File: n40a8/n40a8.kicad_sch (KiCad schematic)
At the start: 92 parts, among them SW1 CPG151101S11-16, SW10 CPG151101S11-16, SW11 CPG151101S11-16, SW12 CPG151101S11-16, SW13 CPG151101S11-16, SW14 CPG151101S11-16, SW15 CPG151101S11-16, SW16 CPG151101S11-16, SW17 CPG151101S11-16, SW18 CPG151101S11-16, SW19 CPG151101S11-16, SW2 CPG151101S11-16, SW20 CPG151101S11-16, SW21 CPG151101S11-16, SW22 CPG151101S11-16, SW23 CPG151101S11-16, SW24 CPG151101S11-16, SW25 CPG151101S11-16, SW26 CPG151101S11-16, SW27 CPG151101S11-16, SW28 CPG151101S11-16, SW29 CPG151101S11-16, SW3 CPG151101S11-16, SW30 CPG151101S11-16, SW31 CPG151101S11-16, SW32 CPG151101S11-16, SW33 CPG151101S11-16, SW34 CPG151101S11-16, SW35 CPG151101S11-16, SW36 CPG151101S11-16, SW37 CPG151101S11-16, SW38 CPG151101S11-16, SW39 CPG151101S11-16, SW4 CPG151101S11-16, SW40 CPG151101S11-16, SW41 CPG151101S11-16, SW42 CPG151101S11-16, SW43 SW_RST, SW44 SW_PWR, SW5 CPG151101S11-16, SW6 CPG151101S11-16, SW7 CPG151101S11-16, SW8 CPG151101S11-16, SW9 CPG151101S11-16, U1 BLE-Micro-Pro-2, U2 TPS61221

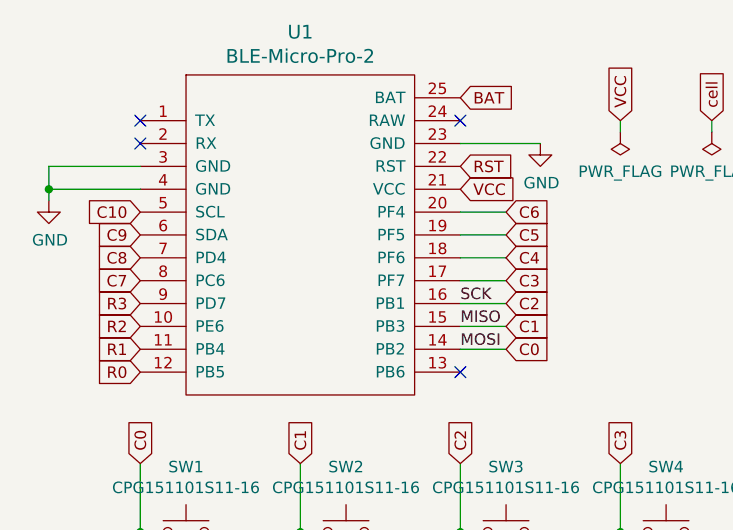
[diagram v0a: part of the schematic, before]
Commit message: revice for PCBA
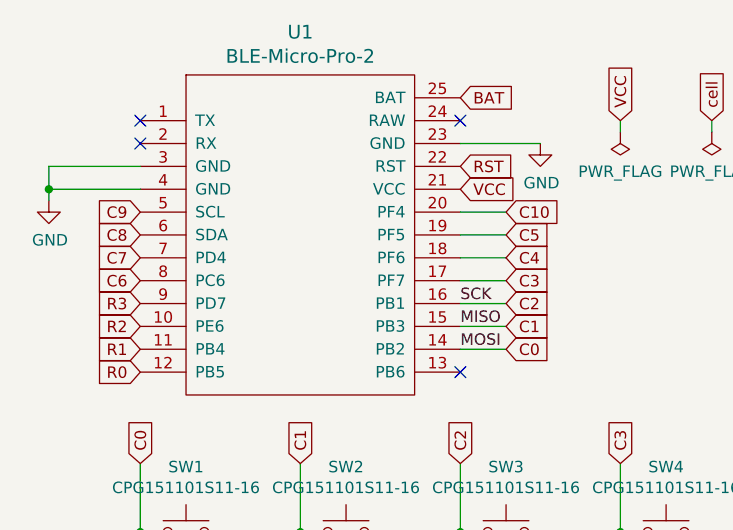
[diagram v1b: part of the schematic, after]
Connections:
- net C10: now also U1.20 (PF4); no longer U1.5 (SCL)
- net C6: now also U1.8 (PC6); no longer U1.20 (PF4)
- net C7: now also U1.7 (PD4); no longer U1.8 (PC6)
- net C8: now also U1.6 (SDA); no longer U1.7 (PD4)
- net C9: now also U1.5 (SCL); no longer U1.6 (SDA)
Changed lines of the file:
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@@
 	(global_label "C9"
 		(shape input)
-		(at 25.4 38.1 180)
-		(effects
-			(font
-				(size 1.27 1.27)
-			)
-			(justify right)
-		)
-		(property "Intersheetrefs" "${INTERSHEET_REFS}"
-			(at 25.4 38.1 0)
+		(at 25.4 35.56 180)
+		(effects
+			(font
+				(size 1.27 1.27)
+			)
+			(justify right)
+		)
+		(property "Intersheetrefs" "${INTERSHEET_REFS}"
+			(at 25.4 35.56 0)
 			(effects
 				(font
@@
 	(global_label "C7"
 		(shape input)
+		(at 25.4 40.64 180)
+		(effects
+			(font
+				(size 1.27 1.27)
+			)
+			(justify right)
+		)
+		(property "Intersheetrefs" "${INTERSHEET_REFS}"
+			(at 25.4 40.64 0)
+			(effects
+				(font
+					(size 1.27 1.27)
+				)
+				(hide yes)
+			)
+		)
+	)
+	(global_label "BAT"
+		(shape input)
+		(at 60.96 22.86 0)
+		(effects
+			(font
+				(size 1.27 1.27)
+			)
+			(justify left)
+		)
+		(property "Intersheetrefs" "${INTERSHEET_REFS}"
+			(at 60.96 22.86 0)
+			(effects
+				(font
+					(size 1.27 1.27)
+				)
+				(hide yes)
+			)
+		)
+	)
+	(global_label "VCC"
+		(shape input)
+		(at 78.74 25.4 90)
+		(effects
+			(font
+				(size 1.27 1.27)
+			)
+			(justify left)
+		)
+		(property "Intersheetrefs" "${INTERSHEET_REFS}"
+			(at 78.74 25.4 0)
+			(effects
+				(font
+					(size 1.27 1.27)
+				)
+				(hide yes)
+			)
+		)
+	)
+	(global_label "C10"
+		(shape input)
+		(at 203.2 63.5 90)
+		(effects
+			(font
+				(size 1.27 1.27)
+			)
+			(justify left)
+		)
+		(property "Intersheetrefs" "${INTERSHEET_REFS}"
+			(at 203.2 63.5 0)
+			(effects
+				(font
+					(size 1.27 1.27)
+				)
+				(hide yes)
+			)
+		)
+	)
+	(global_label "C6"
+		(shape input)
 		(at 25.4 43.18 180)
 		(effects
@@
 		)
 	)
-	(global_label "BAT"
-		(shape input)
-		(at 60.96 22.86 0)
-		(effects
-			(font
-				(size 1.27 1.27)
-			)
-			(justify left)
-		)
-		(property "Intersheetrefs" "${INTERSHEET_REFS}"
-			(at 60.96 22.86 0)
-			(effects
-				(font
-					(size 1.27 1.27)
-				)
-				(hide yes)
-			)
-		)
-	)
-	(global_label "VCC"
-		(shape input)
-		(at 78.74 25.4 90)
-		(effects
-			(font
-				(size 1.27 1.27)
-			)
-			(justify left)
-		)
-		(property "Intersheetrefs" "${INTERSHEET_REFS}"
-			(at 78.74 25.4 0)
+	(global_label "C0"
+		(shape input)
+		(at 66.04 50.8 0)
+		(effects
+			(font
+				(size 1.27 1.27)
+			)
+			(justify left)
+		)
+		(property "Intersheetrefs" "${INTERSHEET_REFS}"
+			(at 66.04 50.8 0)
+			(effects
+				(font
+					(size 1.27 1.27)
+				)
+				(hide yes)
+			)
+		)
+	)
+	(global_label "C5"
+		(shape input)
+		(at 66.04 38.1 0)
+		(effects
+			(font
+				(size 1.27 1.27)
+			)
+			(justify left)
+		)
+		(property "Intersheetrefs" "${INTERSHEET_REFS}"
+			(at 66.04 38.1 0)
+			(effects
+				(font
+					(size 1.27 1.27)
+				)
+				(hide yes)
+			)
+		)
+	)
+	(global_label "cell"
+		(shape input)
+		(at 96.52 172.72 0)
+		(effects
+			(font
+				(size 1.27 1.27)
+			)
+			(justify left)
+		)
+		(property "Intersheetrefs" "${INTERSHEET_REFS}"
+			(at 96.52 172.72 0)
+			(effects
+				(font
+					(size 1.27 1.27)
+				)
+				(hide yes)
+			)
+		)
+	)
+	(global_label "C2"
+		(shape input)
+		(at 66.04 45.72 0)
+		(effects
+			(font
+				(size 1.27 1.27)
+			)
+			(justify left)
+		)
+		(property "Intersheetrefs" "${INTERSHEET_REFS}"
+			(at 66.04 45.72 0)
+			(effects
+				(font
+					(size 1.27 1.27)
+				)
+				(hide yes)
+			)
+		)
+	)
+	(global_label "C5"
+		(shape input)
+		(at 114.3 63.5 90)
+		(effects
+			(font
+				(size 1.27 1.27)
+			)
+			(justify left)
+		)
+		(property "Intersheetrefs" "${INTERSHEET_REFS}"
+			(at 114.3 63.5 0)
+			(effects
+				(font
+					(size 1.27 1.27)
+				)
+				(hide yes)
+			)
+		)
+	)
+	(global_label "C8"
+		(shape input)
+		(at 25.4 38.1 180)
+		(effects
+			(font
+				(size 1.27 1.27)
+			)
+			(justify right)
+		)
+		(property "Intersheetrefs" "${INTERSHEET_REFS}"
+			(at 25.4 38.1 0)
 			(effects
 				(font
@@
 	(global_label "C10"
 		(shape input)
-		(at 203.2 63.5 90)
-		(effects
-			(font
-				(size 1.27 1.27)
-			)
-			(justify left)
-		)
-		(property "Intersheetrefs" "${INTERSHEET_REFS}"
-			(at 203.2 63.5 0)
-			(effects
-				(font
-					(size 1.27 1.27)
-				)
-				(hide yes)
-			)
-		)
-	)
-	(global_label "C6"
-		(shape input)
 		(at 66.04 35.56 0)
 		(effects
@@
 			(effects
 				(font
-					(size 1.27 1.27)
-				)
-				(hide yes)
-			)
-		)
-	)
-	(global_label "C0"
-		(shape input)
-		(at 66.04 50.8 0)
-		(effects
-			(font
-				(size 1.27 1.27)
-			)
-			(justify left)
-		)
-		(property "Intersheetrefs" "${INTERSHEET_REFS}"
-			(at 66.04 50.8 0)
-			(effects
-				(font
-					(size 1.27 1.27)
-				)
-				(hide yes)
-			)
-		)
-	)
-	(global_label "C5"
-		(shape input)
-		(at 66.04 38.1 0)
-		(effects
-			(font
-				(size 1.27 1.27)
-			)
-			(justify left)
-		)
-		(property "Intersheetrefs" "${INTERSHEET_REFS}"
-			(at 66.04 38.1 0)
-			(effects
-				(font
-					(size 1.27 1.27)
-				)
-				(hide yes)
-			)
-		)
-	)
-	(global_label "cell"
-		(shape input)
-		(at 96.52 172.72 0)
-		(effects
-			(font
-				(size 1.27 1.27)
-			)
-			(justify left)
-		)
-		(property "Intersheetrefs" "${INTERSHEET_REFS}"
-			(at 96.52 172.72 0)
-			(effects
-				(font
-					(size 1.27 1.27)
-				)
-				(hide yes)
-			)
-		)
-	)
-	(global_label "C2"
-		(shape input)
-		(at 66.04 45.72 0)
-		(effects
-			(font
-				(size 1.27 1.27)
-			)
-			(justify left)
-		)
-		(property "Intersheetrefs" "${INTERSHEET_REFS}"
-			(at 66.04 45.72 0)
-			(effects
-				(font
-					(size 1.27 1.27)
-				)
-				(hide yes)
-			)
-		)
-	)
-	(global_label "C5"
-		(shape input)
-		(at 114.3 63.5 90)
-		(effects
-			(font
-				(size 1.27 1.27)
-			)
-			(justify left)
-		)
-		(property "Intersheetrefs" "${INTERSHEET_REFS}"
-			(at 114.3 63.5 0)
-			(effects
-				(font
-					(size 1.27 1.27)
-				)
-				(hide yes)
-			)
-		)
-	)
-	(global_label "C8"
-		(shape input)
-		(at 25.4 40.64 180)
-		(effects
-			(font
-				(size 1.27 1.27)
-			)
-			(justify right)
-		)
-		(property "Intersheetrefs" "${INTERSHEET_REFS}"
-			(at 25.4 40.64 0)
-			(effects
-				(font
-					(size 1.27 1.27)
-				)
-				(hide yes)
-			)
-		)
-	)
-	(global_label "C10"
-		(shape input)
-		(at 25.4 35.56 180)
-		(effects
-			(font
-				(size 1.27 1.27)
-			)
-			(justify right)
-		)
-		(property "Intersheetrefs" "${INTERSHEET_REFS}"
-			(at 25.4 35.56 0)
-			(effects
-				(font
